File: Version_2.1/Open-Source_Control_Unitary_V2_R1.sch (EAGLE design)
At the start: 355 parts, among them IC10 MCP6002SMT, IC11 MCP6002SMT, IC12 MCP6002SMT, IC14 MCP6001, IC2 ULN2003AD, IC4 74HC165D, IC5 74HC165D, J24 6p-2.54, K1 JS1-24V-F, K2 JS1-24V-F, K3 JS1-24V-F, K4 JS1-24V-F, K5 JS1-24V-F, Q1 MMBT2907, T4 DA2304-AL, U1 OSD3358-512M-ICB, U16 AT97SC3205T-G3M4400B, U2 TPD4S012_DRY_6_P1_M, U21 S25FL127S, U27 LAN8710, U28 TCAN1051HV, U29 MAX3483EESA+T, U4 APX811-31UGSOT, U40 ISO3086TDW, U5 TLVH431, U6 SN74LVC2G241_DCU_8, X1 10118194-0001LF, X10 MC4, X11 MC4, X12 MC4, X2 J0011D01BNL, X21 MC10, X24 MSTBA2, X3 MC4, X31 MC4, X4 CTI-JTAG, X41 MSTBA3, X5 DM3CS-SF, X6 6p-2.54, X7 TH-2X10, Y7 7A-25.000MAAE-T

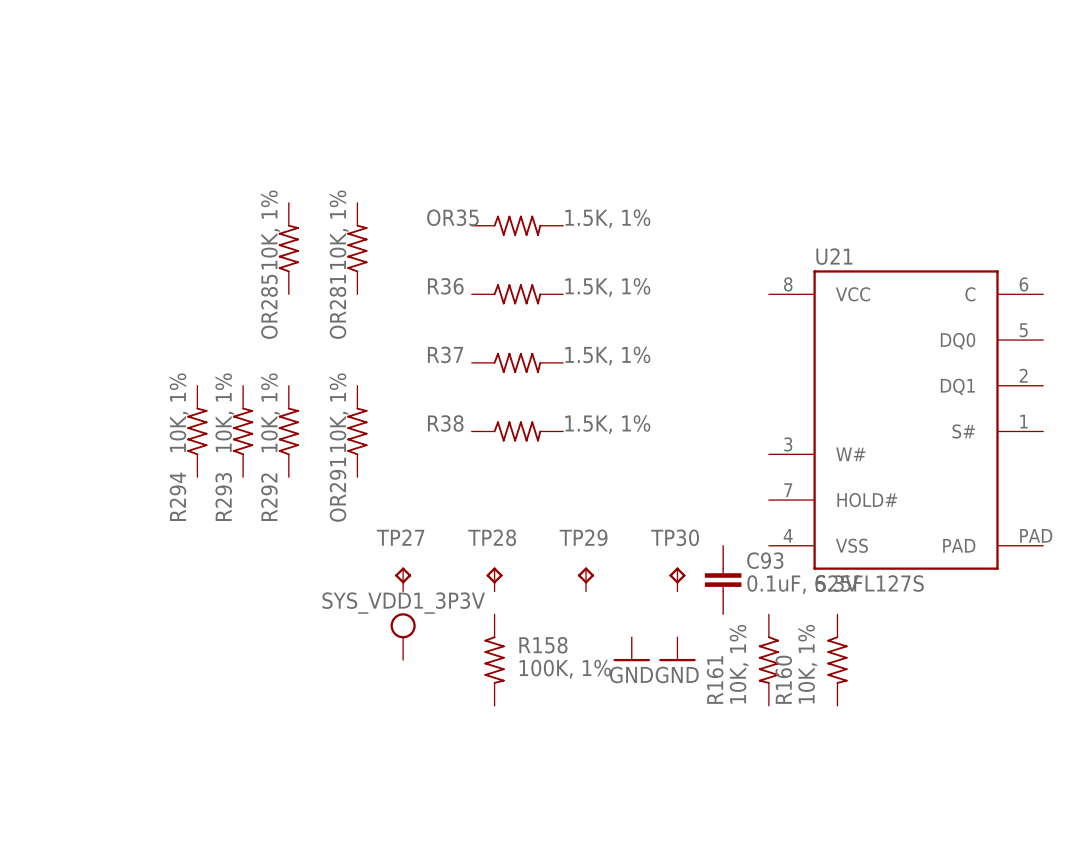
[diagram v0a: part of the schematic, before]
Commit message: Add files via upload
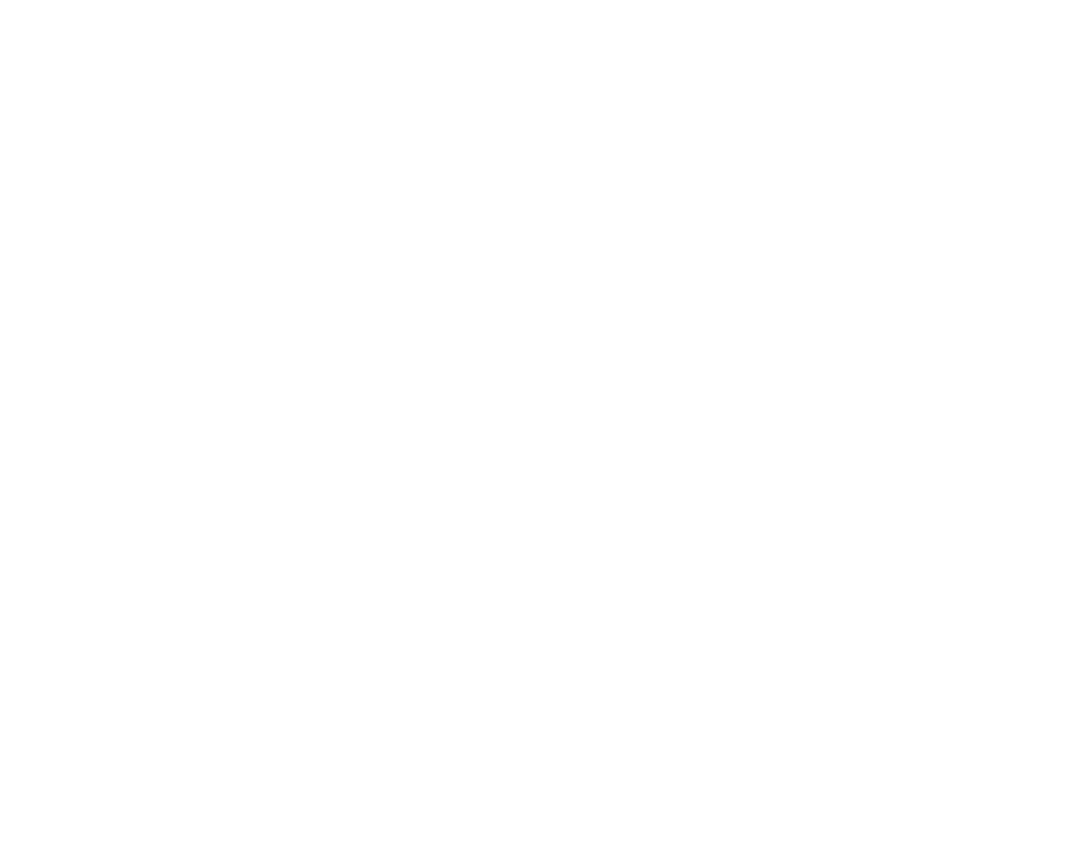
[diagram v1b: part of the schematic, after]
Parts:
- removed C93: 0.1uF, 6.3V, OSD3358-SM-RED Platform:CC0402
- removed OR281, OR285, OR291, R160, R161, R292, R293, R294: 10K, 1%, OSD3358-SM-RED Platform:R-US_R0402
- removed OR35, R36, R37, R38: 1.5K, 1%, OSD3358-SM-RED Platform:R-US_R0402
- removed R158: 100K, 1%, OSD3358-SM-RED Platform:R-US_R0402
- removed TP27, TP28, TP29, TP30: TPB0,65, OSD3358-SM-RED Platform:TPB0,65
- removed U21: S25FL127S, OSD3358-SM-RED Platform:S25FL127S
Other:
- note removed: "There are many footprint compatible (8-WSON) parts for the NOR flash if the listed part is not available."
